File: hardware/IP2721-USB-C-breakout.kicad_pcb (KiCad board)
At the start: 2 copper layers, 100 x 100 mm, 13 parts, among them J1 Conn_01x02_Female, Q1 AO3400A, U1 IP2721, U2 USB_C_PD_CONNECTOR

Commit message: update and test,
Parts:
- C1: value C106,0805 -> C105,0805,50V
- C2: value C105,0805 -> C106,0805,50V
- R1, R2: value R513,0805 -> R512,0805
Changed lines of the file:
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@@
       (linewidth 0.100000)
       (plotframeref false)
-      (viasonmask false)
+      (viasonmask true)
       (mode 1)
       (useauxorigin false)
@@
       (outputformat 1)
       (mirror false)
-      (drillshape 1)
+      (drillshape 0)
       (scaleselection 1)
-      (outputdirectory ""))
+      (outputdirectory "gerber/"))
   )
   (net 0 "")
@@
     (add_net GND)
     (add_net "Net-(Q1-PadG)")
+    (add_net "Net-(U1-Pad10)")
+    (add_net "Net-(U1-Pad14)")
+    (add_net "Net-(U1-Pad15)")
+    (add_net "Net-(U1-Pad3)")
+    (add_net "Net-(U1-Pad4)")
+    (add_net "Net-(U1-Pad6)")
+    (add_net "Net-(U1-Pad7)")
+    (add_net "Net-(U1-Pad8)")
+    (add_net "Net-(U1-Pad9)")
     (add_net "Net-(U2-PadS1)")
     (add_net SEL)
@@
     (fp_text value USB_C_PD_CONNECTOR (at 0 6) (layer F.Fab)
       (effects (font (size 1 1) (thickness 0.15)))
-    )
-    (fp_text user REF* (at 0 0) (layer F.Fab)
-      (effects (font (size 1 1) (thickness 0.1)))
     )
     (fp_line (start -5 5.15) (end 5 5.15) (layer F.CrtYd) (width 0.12))
@@
     (fp_line (start 4.47 -3.425) (end 4.47 4.525) (layer F.Fab) (width 0.12))
     (fp_line (start -4.47 -3.425) (end 4.47 -3.425) (layer F.Fab) (width 0.12))
+    (fp_text user REF* (at 0 0) (layer F.Fab)
+      (effects (font (size 1 1) (thickness 0.1)))
+    )
     (pad S1 thru_hole oval (at -4.32 1.87 180) (size 1 1.6) (drill oval 0.6 1.2) (layers *.Cu *.Mask)
       (net 6 "Net-(U2-PadS1)"))
@@
       (effects (font (size 0.5 0.5) (thickness 0.08)))
     )
-    (pad 2 smd roundrect (at 1 0 90) (size 1.2 1.4) (layers F.Cu F.Paste F.Mask) (roundrect_rratio 0.208333)
+    (pad 2 smd roundrect (at 1 0 90) (size 1.2 1.4) (layers F.Cu F.Paste F.Mask) (roundrect_rratio 0.2083325)
       (net 5 SEL))
-    (pad 1 smd roundrect (at -1 0 90) (size 1.2 1.4) (layers F.Cu F.Paste F.Mask) (roundrect_rratio 0.208333)
+    (pad 1 smd roundrect (at -1 0 90) (size 1.2 1.4) (layers F.Cu F.Paste F.Mask) (roundrect_rratio 0.2083325)
       (net 2 VIN))
     (model ${KISYS3DMOD}/Resistor_SMD.3dshapes/R_0805_2012Metric.wrl
@@
       (effects (font (size 1 1) (thickness 0.15)))
     )
-    (fp_text value R513,0805 (at 0 1.65) (layer F.Fab)
+    (fp_text value R512,0805 (at 0 1.65) (layer F.Fab)
       (effects (font (size 1 1) (thickness 0.15)))
     )
@@
       (effects (font (size 0.5 0.5) (thickness 0.08)))
     )
-    (pad 2 smd roundrect (at 1 0 180) (size 1.2 1.4) (layers F.Cu F.Paste F.Mask) (roundrect_rratio 0.208333)
-      (net 1 GND))
-    (pad 1 smd roundrect (at -1 0 180) (size 1.2 1.4) (layers F.Cu F.Paste F.Mask) (roundrect_rratio 0.208333)
+    (pad 2 smd roundrect (at 1 0 180) (size 1.2 1.4) (layers F.Cu F.Paste F.Mask) (roundrect_rratio 0.2083325)
+      (net 1 GND))
+    (pad 1 smd roundrect (at -1 0 180) (size 1.2 1.4) (layers F.Cu F.Paste F.Mask) (roundrect_rratio 0.2083325)
       (net 8 CC2))
     (model ${KISYS3DMOD}/Resistor_SMD.3dshapes/R_0805_2012Metric.wrl
@@
       (effects (font (size 1 1) (thickness 0.15)))
     )
-    (fp_text value R513,0805 (at 0 1.65) (layer F.Fab)
+    (fp_text value R512,0805 (at 0 1.65) (layer F.Fab)
       (effects (font (size 1 1) (thickness 0.15)))
     )
@@
       (effects (font (size 0.5 0.5) (thickness 0.08)))
     )
-    (pad 2 smd roundrect (at 1 0 180) (size 1.2 1.4) (layers F.Cu F.Paste F.Mask) (roundrect_rratio 0.208333)
-      (net 1 GND))
-    (pad 1 smd roundrect (at -1 0 180) (size 1.2 1.4) (layers F.Cu F.Paste F.Mask) (roundrect_rratio 0.208333)
+    (pad 2 smd roundrect (at 1 0 180) (size 1.2 1.4) (layers F.Cu F.Paste F.Mask) (roundrect_rratio 0.2083325)
+      (net 1 GND))
+    (pad 1 smd roundrect (at -1 0 180) (size 1.2 1.4) (layers F.Cu F.Paste F.Mask) (roundrect_rratio 0.2083325)
       (net 4 CC1))
     (model ${KISYS3DMOD}/Resistor_SMD.3dshapes/R_0805_2012Metric.wrl
@@
       (effects (font (size 1 1) (thickness 0.15)))
     )
-    (fp_text value C105,0805 (at 0 1.68) (layer F.Fab)
+    (fp_text value C106,0805,50V (at 0 1.68) (layer F.Fab)
       (effects (font (size 1 1) (thickness 0.15)))
     )
@@
       (effects (font (size 0.5 0.5) (thickness 0.08)))
     )
-    (pad 2 smd roundrect (at 1.0375 0) (size 1.175 1.45) (layers F.Cu F.Paste F.Mask) (roundrect_rratio 0.212766)
-      (net 1 GND))
-    (pad 1 smd roundrect (at -1.0375 0) (size 1.175 1.45) (layers F.Cu F.Paste F.Mask) (roundrect_rratio 0.212766)
+    (pad 2 smd roundrect (at 1.0375 0) (size 1.175 1.45) (layers F.Cu F.Paste F.Mask) (roundrect_rratio 0.2127659574468085)
+      (net 1 GND))
+    (pad 1 smd roundrect (at -1.0375 0) (size 1.175 1.45) (layers F.Cu F.Paste F.Mask) (roundrect_rratio 0.2127659574468085)
       (net 3 VOUT))
     (model ${KISYS3DMOD}/Capacitor_SMD.3dshapes/C_0805_2012Metric.wrl
@@
       (effects (font (size 1 1) (thickness 0.15)))
     )
-    (fp_text value C106,0805 (at 0 1.68) (layer F.Fab)
+    (fp_text value C105,0805,50V (at 0 1.68) (layer F.Fab)
       (effects (font (size 1 1) (thickness 0.15)))
     )
@@
       (effects (font (size 0.5 0.5) (thickness 0.08)))
     )
-    (pad 2 smd roundrect (at 1.0375 0) (size 1.175 1.45) (layers F.Cu F.Paste F.Mask) (roundrect_rratio 0.212766)
-      (net 1 GND))
-    (pad 1 smd roundrect (at -1.0375 0) (size 1.175 1.45) (layers F.Cu F.Paste F.Mask) (roundrect_rratio 0.212766)
+    (pad 2 smd roundrect (at 1.0375 0) (size 1.175 1.45) (layers F.Cu F.Paste F.Mask) (roundrect_rratio 0.2127659574468085)
+      (net 1 GND))
+    (pad 1 smd roundrect (at -1.0375 0) (size 1.175 1.45) (layers F.Cu F.Paste F.Mask) (roundrect_rratio 0.2127659574468085)
       (net 2 VIN))
     (model ${KISYS3DMOD}/Capacitor_SMD.3dshapes/C_0805_2012Metric.wrl

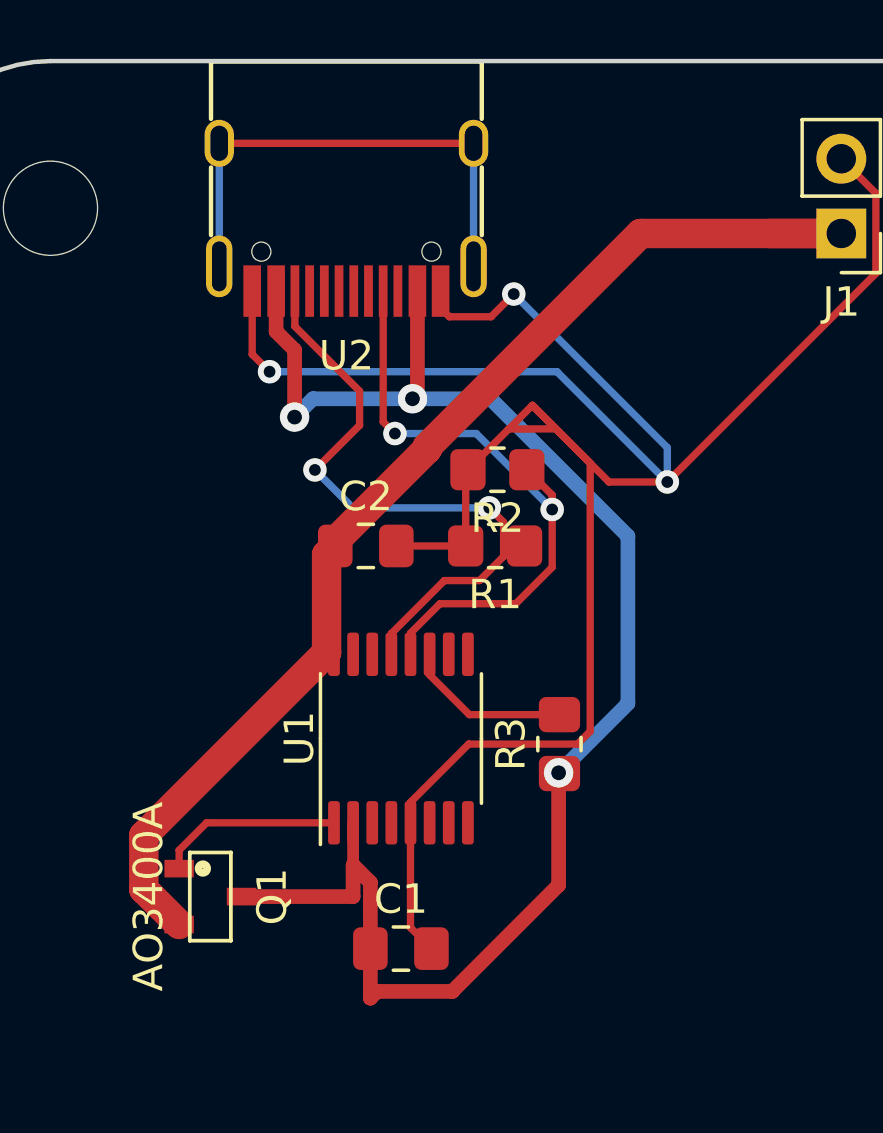
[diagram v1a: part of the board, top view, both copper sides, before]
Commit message: update,
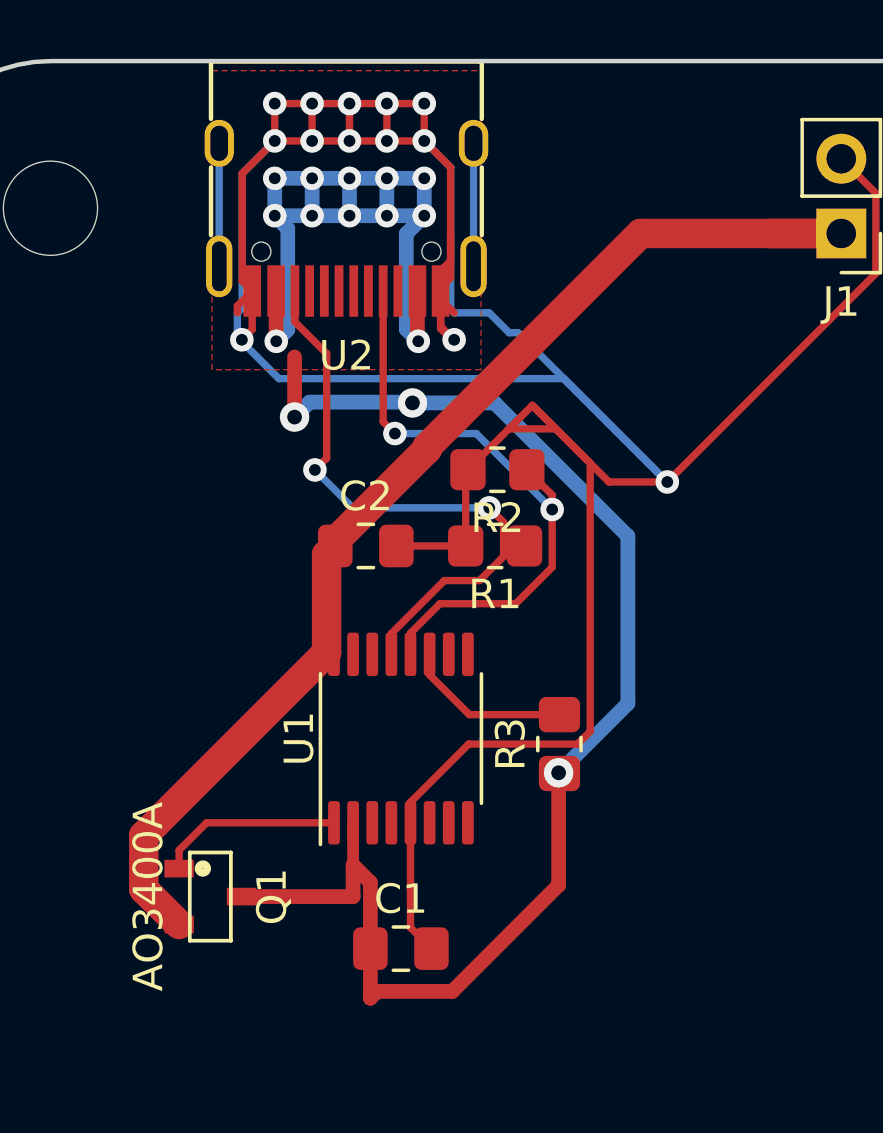
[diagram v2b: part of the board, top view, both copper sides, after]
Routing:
- net GND: track 84.5 -> 131.0 mm, vias 3 -> 13
- net VIN: track 53.7 -> 76.8 mm, vias 3 -> 15
- net Net-(U2-PadS1): track 17.0 -> 8.36 mm
- net CC1: track 22.2 -> 21.3 mm
- added copper zone on F.Cu, net GND
